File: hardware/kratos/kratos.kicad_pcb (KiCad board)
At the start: 4 copper layers, 23.1 x 32.8 mm, 16 parts, among them J1 IO Header, J3 Power Terminal, J4 VIN, U1 AP2138, U3 MIC29310-5.0, U4 DS2745U

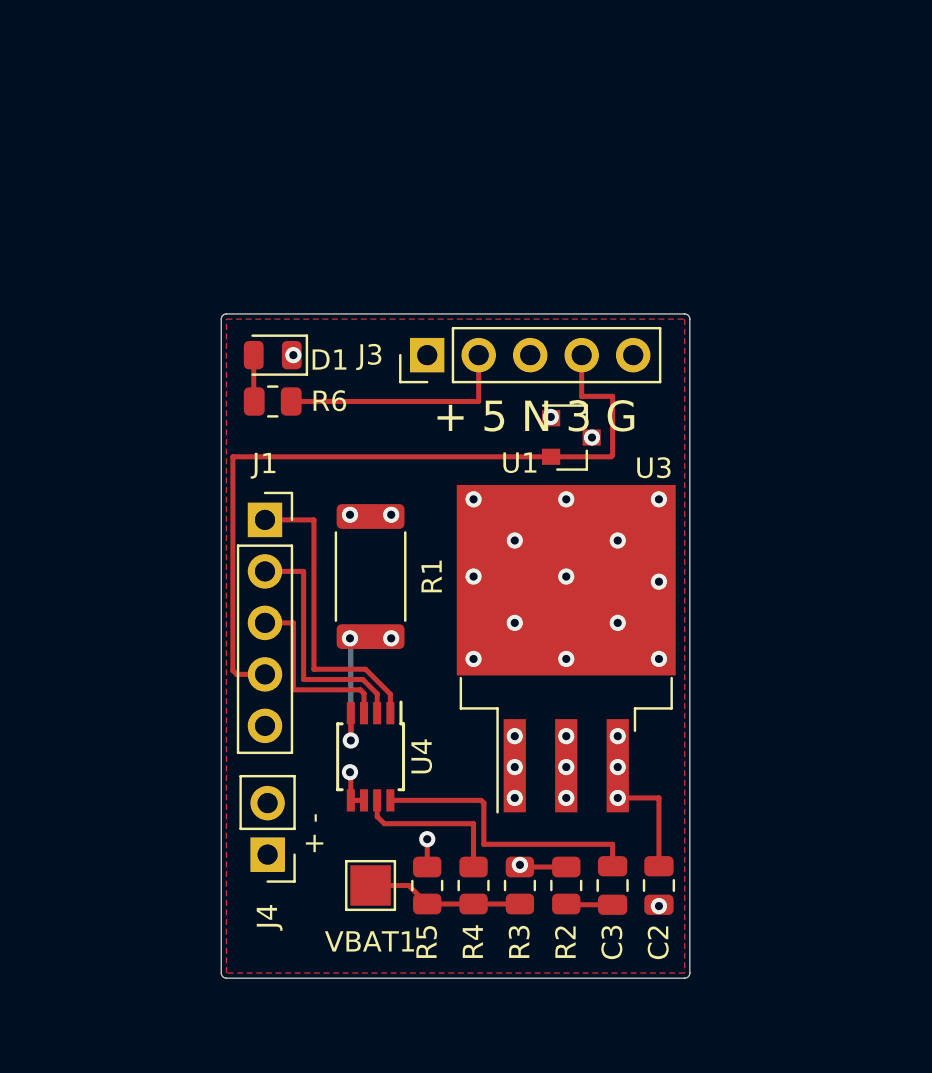
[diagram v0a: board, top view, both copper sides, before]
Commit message: REV C
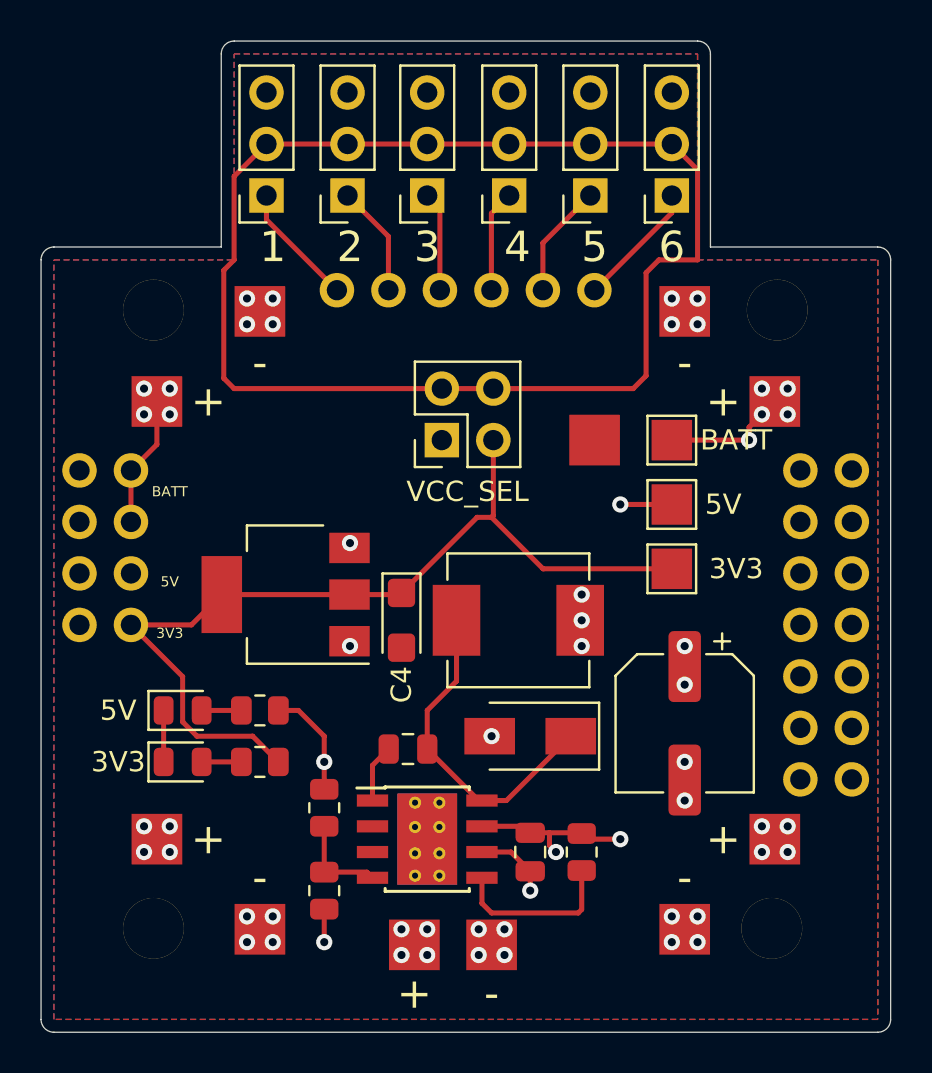
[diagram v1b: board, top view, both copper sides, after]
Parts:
- removed J3: Power Terminal, Connector_PinHeader_2.54mm:PinHeader_1x05_P2.54mm_Vertical
- removed J4: VIN, Connector_PinHeader_2.54mm:PinHeader_1x02_P2.54mm_Vertical
- removed R6: 200, Resistor_SMD:R_0805_2012Metric
- removed U4: DS2745U, Package_SO:TSSOP-8_3x3mm_P0.65mm
- removed VBAT1: DIV_TP, TestPoint:TestPoint_Pad_2.0x2.0mm
- added ?: , , F.Cu at (126.6, 112.3)
- added ?: , , F.Cu at (148.2, 92.6)
- added ?: , , F.Cu at (131.7, 86.2)
- added ?: , , F.Cu at (152.7, 116.7)
- added ?: , , F.Cu at (126.6, 90.7)
- added ?: , , F.Cu at (157.1, 112.3)
- added C1: 10uF, Capacitor_SMD:C_0805_2012Metric, F.Cu at (145.0, 112.9)
- added C4: 22uF, Capacitor_Tantalum_SMD:CP_EIA-3216-18_Kemet-A, F.Cu at (138.7, 101.5)
- added D2: 5V, LED_SMD:LED_0805_2012Metric, F.Cu at (127.9, 105.9)
- added D3: 3V3, LED_SMD:LED_0805_2012Metric, F.Cu at (127.9, 108.5)
- added J10: PWM4, Connector_PinSocket_2.54mm:PinSocket_1x03_P2.54mm_Vertical, F.Cu at (144.0, 80.5)
- added J11: PWM5, Connector_PinSocket_2.54mm:PinSocket_1x03_P2.54mm_Vertical, F.Cu at (148.0, 80.5)
- added J12: PWM6, Connector_PinSocket_2.54mm:PinSocket_1x03_P2.54mm_Vertical, F.Cu at (152.0, 80.5)
- added J6: VCC_SEL, Connector_PinSocket_2.54mm:PinSocket_2x02_P2.54mm_Vertical, F.Cu at (140.7, 92.6)
- added J7: PWM1, Connector_PinSocket_2.54mm:PinSocket_1x03_P2.54mm_Vertical, F.Cu at (132.0, 80.5)
- added J8: PWM2, Connector_PinSocket_2.54mm:PinSocket_1x03_P2.54mm_Vertical, F.Cu at (136.0, 80.5)
- added J9: PWM3, Connector_PinSocket_2.54mm:PinSocket_1x03_P2.54mm_Vertical, F.Cu at (140.0, 80.5)
- added L1: 15uH, inductors:MWSA0603S-150MT, F.Cu at (144.4, 101.5)
- added REF**: XT60, drone:XT60, F.Cu at (131.7, 116.7)
- added REF**: XT60, drone:XT60, F.Cu at (157.1, 90.7)
- added REF**: XT60, drone:XT60, F.Cu at (152.7, 86.2)
- added TP1: BATT, TestPoint:TestPoint_Pad_2.0x2.0mm, F.Cu at (152.0, 92.6)
- added TP2: 5V, TestPoint:TestPoint_Pad_2.0x2.0mm, F.Cu at (152.0, 95.8)
- added TP3: 3V3, TestPoint:TestPoint_Pad_2.0x2.0mm, F.Cu at (152.0, 98.9)
- added U2: AMS1117-3.3, Package_TO_SOT_SMD:SOT-223-3_TabPin2, F.Cu at (133.0, 100.2)
- C2: value 10uF, 16V -> 10nF
- C3: value 10nF -> 220uF; footprint Capacitor_SMD:C_0805_2012Metric -> Capacitor_SMD:CP_Elec_6.3x5.4
- D1: value PWR_5V -> B340A; footprint LED_SMD:LED_0805_2012Metric -> Diode_SMD:D_SMA
- J1: value IO Header -> BATT; footprint Connector_PinSocket_2.54mm:PinSocket_1x05_P2.54mm_Vertical -> drone:XT60
- R1: value 10m -> 10k; footprint Resistor_SMD:R_2512_6332Metric -> Resistor_SMD:R_0805_2012Metric
- R2: value 500 -> 10k
- R3: value 20k -> 3.24k
- R4: value 10k -> 330
- R5: value 4.7k -> 200
- U1: value AP2138 -> TPS5430DDA; footprint Package_TO_SOT_SMD:SOT-23 -> Package_SO:TI_SO-PowerPAD-8_ThermalVias
- U3: value MIC29310-5.0 -> ICARUS SHIELD; footprint Package_TO_SOT_SMD:TO-263-3_TabPin2 -> icarus:icarus-shield
- moved D1 22.7 mm to (145.0, 107.2)
- moved U1 21.0 mm to (140.0, 112.3)
- moved U3 19.6 mm to (141.8, 83.9), turned to 0 degrees
- moved J1 18.1 mm to (140.6, 112.4)
- moved R1 17.1 mm to (147.6, 112.9), turned to -90 degrees
- moved C2 14.1 mm to (139.0, 107.8), turned to 0 degrees
- moved R4 13.6 mm to (131.7, 105.9), turned to 180 degrees
- moved R2 12.5 mm to (134.9, 110.7)
- moved R5 10.3 mm to (131.7, 108.5), turned to 180 degrees
- moved R3 9.66 mm to (134.9, 114.8), turned to 90 degrees
- moved C3 8.76 mm to (152.7, 106.6), turned to -90 degrees
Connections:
- C2 pad 1: +5V -> Net-(C2-Pad1)
- C2 pad 2: GND -> Net-(C2-Pad2)
- C3 pad 1: Net-(C3-Pad1) -> +5V
- C3 pad 2: Net-(C3-Pad2) -> GND
- D1 pad 1: GND -> Net-(C2-Pad2)
- D1 pad 2: Net-(D1-Pad2) -> GND
- J1 pad 1: /scl -> +BATT
- J1 pad 2: /sda -> GND
- R1 pad 1: /Input/rsense+ -> +BATT
- R1 pad 2: GND -> Net-(R1-Pad2)
- R2 pad 1: VDC -> +5V
- R2 pad 2: Net-(C3-Pad1) -> Net-(R2-Pad2)
- R3 pad 1: VDC -> GND
- R3 pad 2: Net-(R3-Pad2) -> Net-(R2-Pad2)
- R4 pad 1: Net-(R3-Pad2) -> +5V
- R5 pad 1: Net-(R3-Pad2) -> +3V3
- R5 pad 2: GND -> Net-(D3-Pad2)
- U1 pad 1: GND -> Net-(C2-Pad1)
- U1 pad 2: +3V3 -> unconnected-(U1-Pad2)
- U1 pad 3: +5V -> unconnected-(U1-Pad3)
- U3 pad 1: VDC -> GND
- U3 pad 2: GND -> +BATT
- U3 pad 3: +5V -> GND
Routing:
- net VCC: track 0.00 -> 67.9 mm
- net +BATT: track 0.00 -> 20.9 mm, vias 0 -> 23
- net Net-(C2-Pad2): track 0.00 -> 16.4 mm
- net /scl: track 15.0 -> 0.00 mm
- net Net-(C3-Pad2): track 14.1 -> 0.00 mm
- net /sda: track 12.1 -> 0.00 mm
- net /p1: track 9.23 -> 0.00 mm
- net +5V: track 16.9 -> 7.95 mm, vias 4 -> 8
- net Net-(R1-Pad2): track 0.00 -> 8.37 mm
- net Net-(R3-Pad2): track 7.74 -> 0.00 mm
- net +3V3: track 37.4 -> 45.2 mm
- net /Input/rsense+: track 6.40 -> 0.00 mm, vias 3 -> 0
- net /pwm6: track 0.00 -> 6.25 mm
- net /pwm1: track 0.00 -> 6.11 mm
- net Net-(D2-Pad2): track 7.84 -> 1.96 mm
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- added copper zone on In1.Cu, net +5V
- added copper zone on In1.Cu, net +BATT
- added copper zone on B.Cu, net GND
- added copper zone on F.Cu, net GND
- added copper zone on In2.Cu, net GND
- removed copper zone on F.Cu, net (none)
- removed copper zone on PWR, net +5V
- removed copper zone on PWR, net /Input/rsense+
- removed copper zone on GND, net GND
- removed copper zone on PWR, net VDC
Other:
- board size 23.1 x 32.8 mm -> 41.9 x 48.9 mm
- net class Default removed
- board text added: "+"
- board text added: "-"
- board text added: "1"
- board text added: "2"
- board text added: "3"
- board text added: "3V3"
- board text added: "4"
- board text added: "5"
- board text added: "5V"
- board text added: "6"
- board text added: "BATT"
- board text added: "kratos :: REV C nnarain"
- board text removed: "+ -"
- board text removed: "+ 5 N 3 G"
- board text removed: "kratos-pdb :: Rev B nnarain"
